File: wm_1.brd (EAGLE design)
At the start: 110.3 x 34 mm, 22 parts, among them T1 MMBT3904, T2 BT138-V, X1 22-23-2031

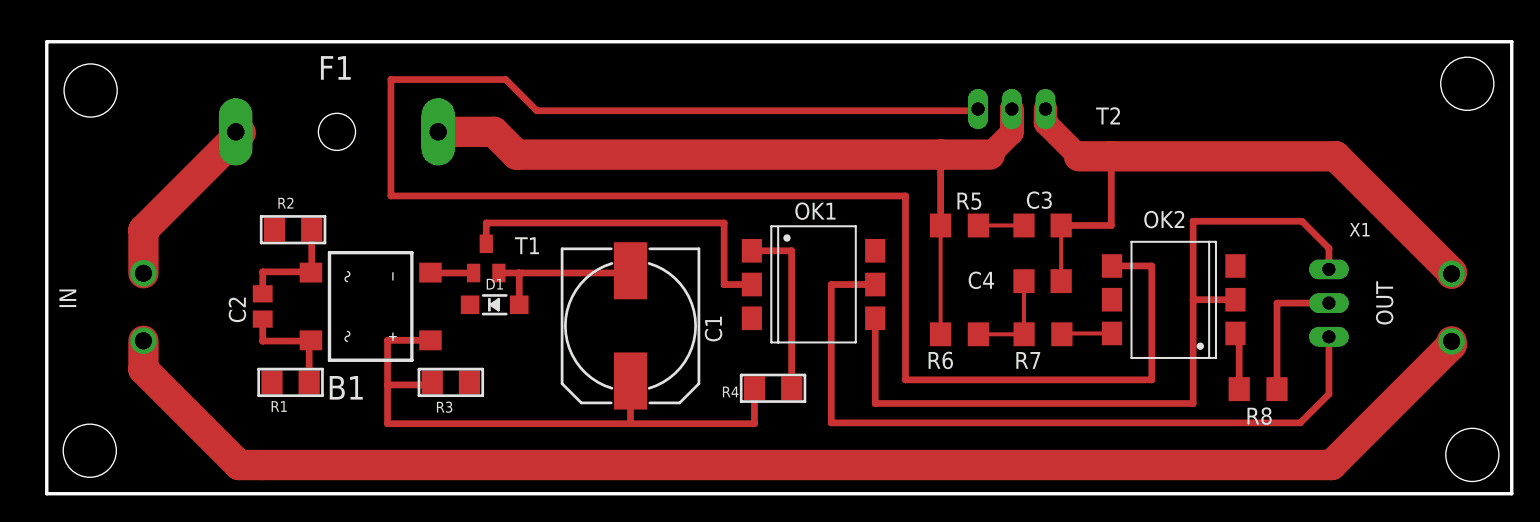
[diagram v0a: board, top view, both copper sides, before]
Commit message: v2.1
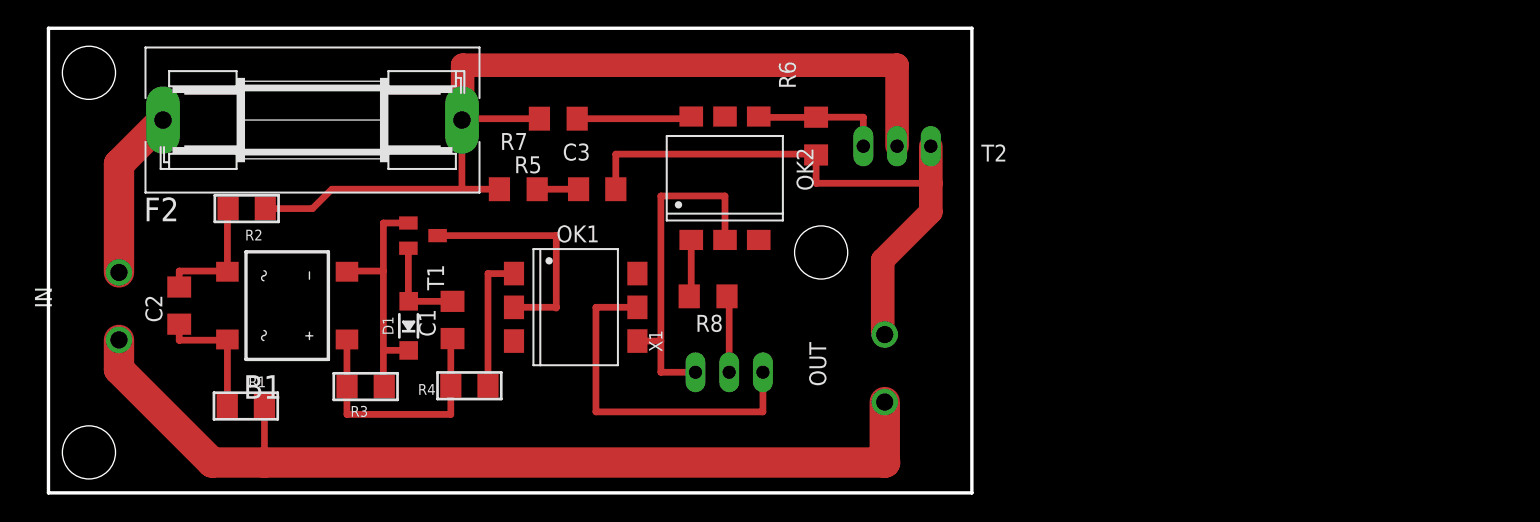
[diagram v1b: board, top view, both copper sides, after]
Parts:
- removed C4: 0.05, rcl:C1206
- removed F1: (no value), fuse:GSH15
- added F2: (no value), fuse:SH22,5A
- C1: value 10uF 10V -> 10 uF 10V; device rcl:140CLH-1010 -> rcl:C1206
- C2: device rcl:C0805 -> rcl:C1206
- R6: value 470 -> 330
- R7: value 360 -> 380
- R8: value 1k -> 470
- moved X1 45.4 mm to (51.4, 9.14), turned to 0 degrees
- moved OUT 42.9 mm to (63.1, 9.46)
- moved R8 42.0 mm to (49.8, 14.9)
- moved R7 39.9 mm to (38.5, 28.2)
- moved OK2 35.0 mm to (51.1, 23.7), turned to 0 degrees
- moved C3 33.6 mm to (41.4, 22.9)
- moved R5 33.3 mm to (35.5, 22.9)
- moved R4 22.9 mm to (31.8, 8.13)
- moved R6 18.4 mm to (57.9, 26.9), turned to 90 degrees
- moved OK1 18.0 mm to (39.8, 14.0)
- moved C1 13.4 mm to (30.5, 13.1), turned to 90 degrees
- moved T2 9.08 mm to (64.0, 28.7)
- moved D1 6.67 mm to (27.2, 12.6), turned to 90 degrees
- moved R3 6.42 mm to (24.0, 8.06)
- moved B1 6.29 mm to (18.1, 14.2)
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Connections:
- removed net N$8: C4.1, R6.2, R7.1
- removed net N$9: F1.2, IN.1, R2.1
- new net FAZA: F2.1, IN.1
- net GATE: now also R6.2
- net HOT: now also F2.2, R2.1, R7.1; no longer F1.1, R6.1
- net LOAD: now also R6.1; no longer C4.2
- net N$3: now also C1.2; no longer C1.-
- net N$5: now also C1.1; no longer C1.+
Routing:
- net GATE: track 136.8 -> 10.1 mm
- net GROUND: track 107.7 -> 71.6 mm
- net GND: track 59.9 -> 26.2 mm
- net ZERO: track 56.4 -> 26.6 mm
- net N$5: track 47.9 -> 19.5 mm
- net N$4: track 3.90 -> 19.2 mm
- net N$9: track 13.6 -> 0.00 mm
- net FAZA: track 0.00 -> 12.8 mm
- net HOT: track 61.5 -> 72.4 mm
- net N$7: track 26.2 -> 17.6 mm
- net N$8: track 7.45 -> 0.00 mm
- net N$3: track 14.3 -> 7.34 mm
- net LOAD: track 49.6 -> 44.3 mm
- net N$16: track 3.80 -> 8.75 mm
- net ON/OFF: track 10.4 -> 5.88 mm
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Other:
- board size 110.3 x 34 mm -> 69.5 x 35 mm

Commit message: v2.2
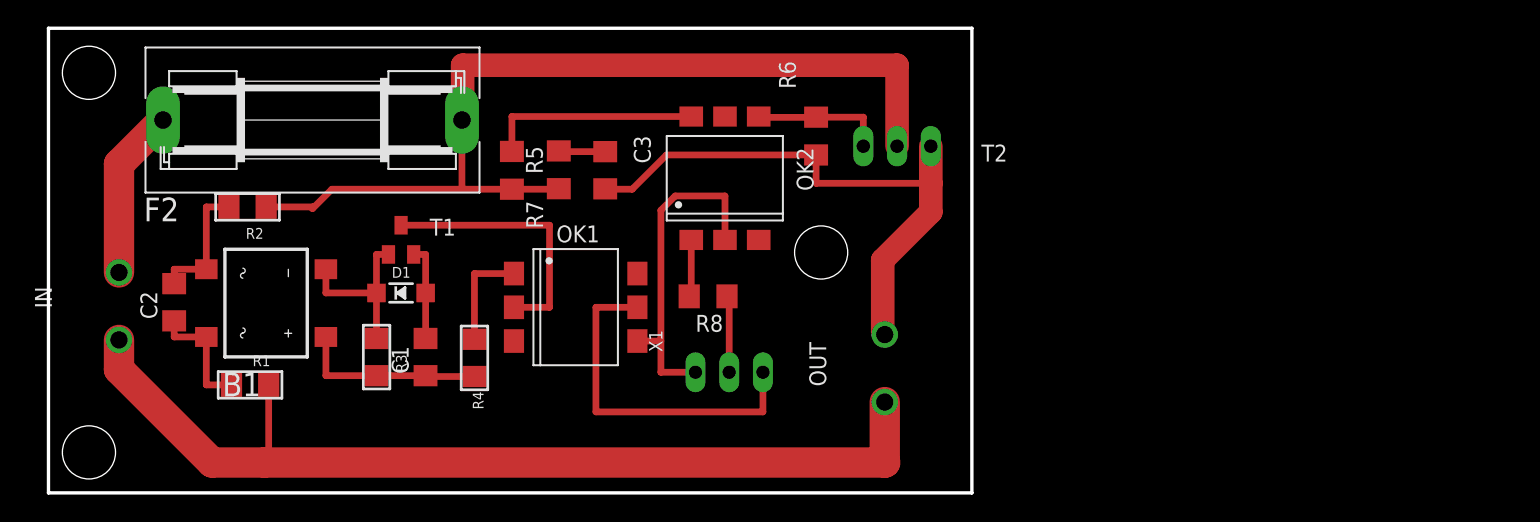
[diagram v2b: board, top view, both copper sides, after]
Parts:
- moved R7 5.22 mm to (35.0, 24.3), turned to 90 degrees
- moved C1 3.45 mm to (28.5, 10.3)
- moved R5 3.38 mm to (38.5, 24.4), turned to 270 degrees
- moved D1 2.54 mm to (26.7, 15.1), turned to 0 degrees
- moved R3 2.37 mm to (24.8, 10.3), turned to 270 degrees
- moved R4 2.13 mm to (32.2, 10.2), turned to 270 degrees
- moved T1 1.68 mm to (26.7, 19.1), turned to 0 degrees
- moved R1 1.62 mm to (15.3, 8.19)
- moved B1 1.60 mm to (16.5, 14.4)
- moved C3 1.55 mm to (42.0, 24.4), turned to 270 degrees
- moved C2 0.46 mm to (9.59, 14.4)
- moved R2 0.14 mm to (15.1, 21.6)
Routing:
- net N$16: track 8.75 -> 16.4 mm
- net N$4: track 19.2 -> 13.1 mm
- net N$5: track 19.5 -> 14.2 mm
- net GROUND: track 71.6 -> 75.1 mm
- net N$6: track 10.4 -> 7.93 mm
- net N$7: track 17.6 -> 20.0 mm
- net HOT: track 72.4 -> 71.0 mm
- net LOAD: track 44.3 -> 43.5 mm
- net N$1: track 10.5 -> 9.76 mm
- net GND: track 26.2 -> 25.6 mm
